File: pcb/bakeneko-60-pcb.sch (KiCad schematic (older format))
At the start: 17 parts, among them J1 JST SH 4-pin, SW1 Reset, U1 USBLC6-2SC6, U2 ATmega32U4-AU, Y1 16MHz

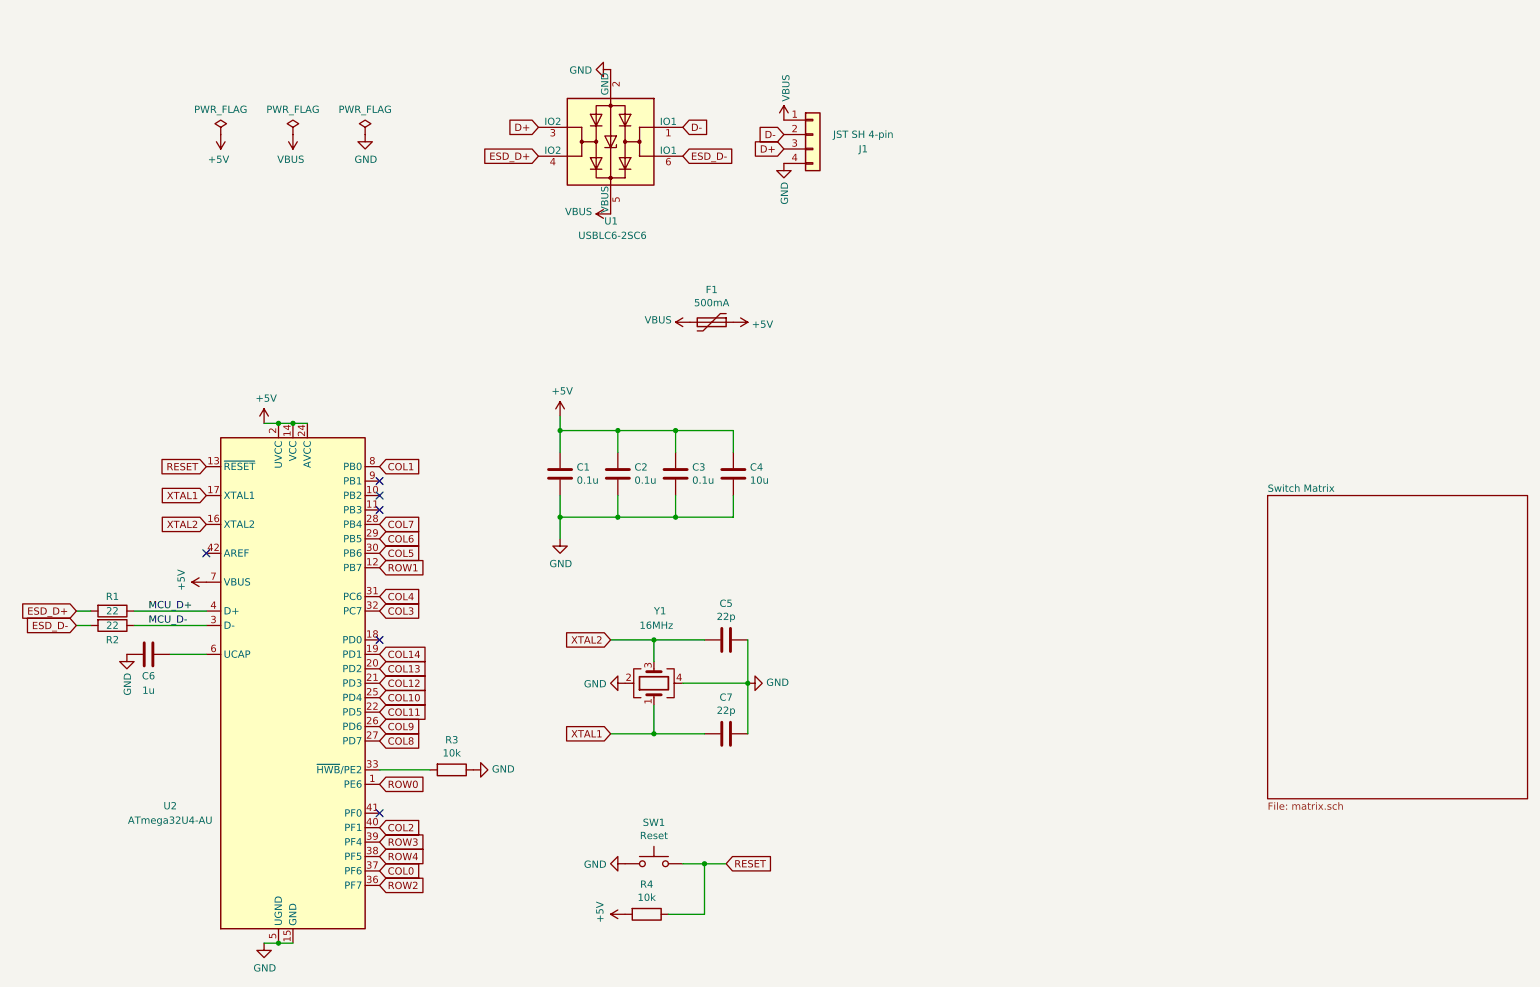
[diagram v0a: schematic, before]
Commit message: Update PCB
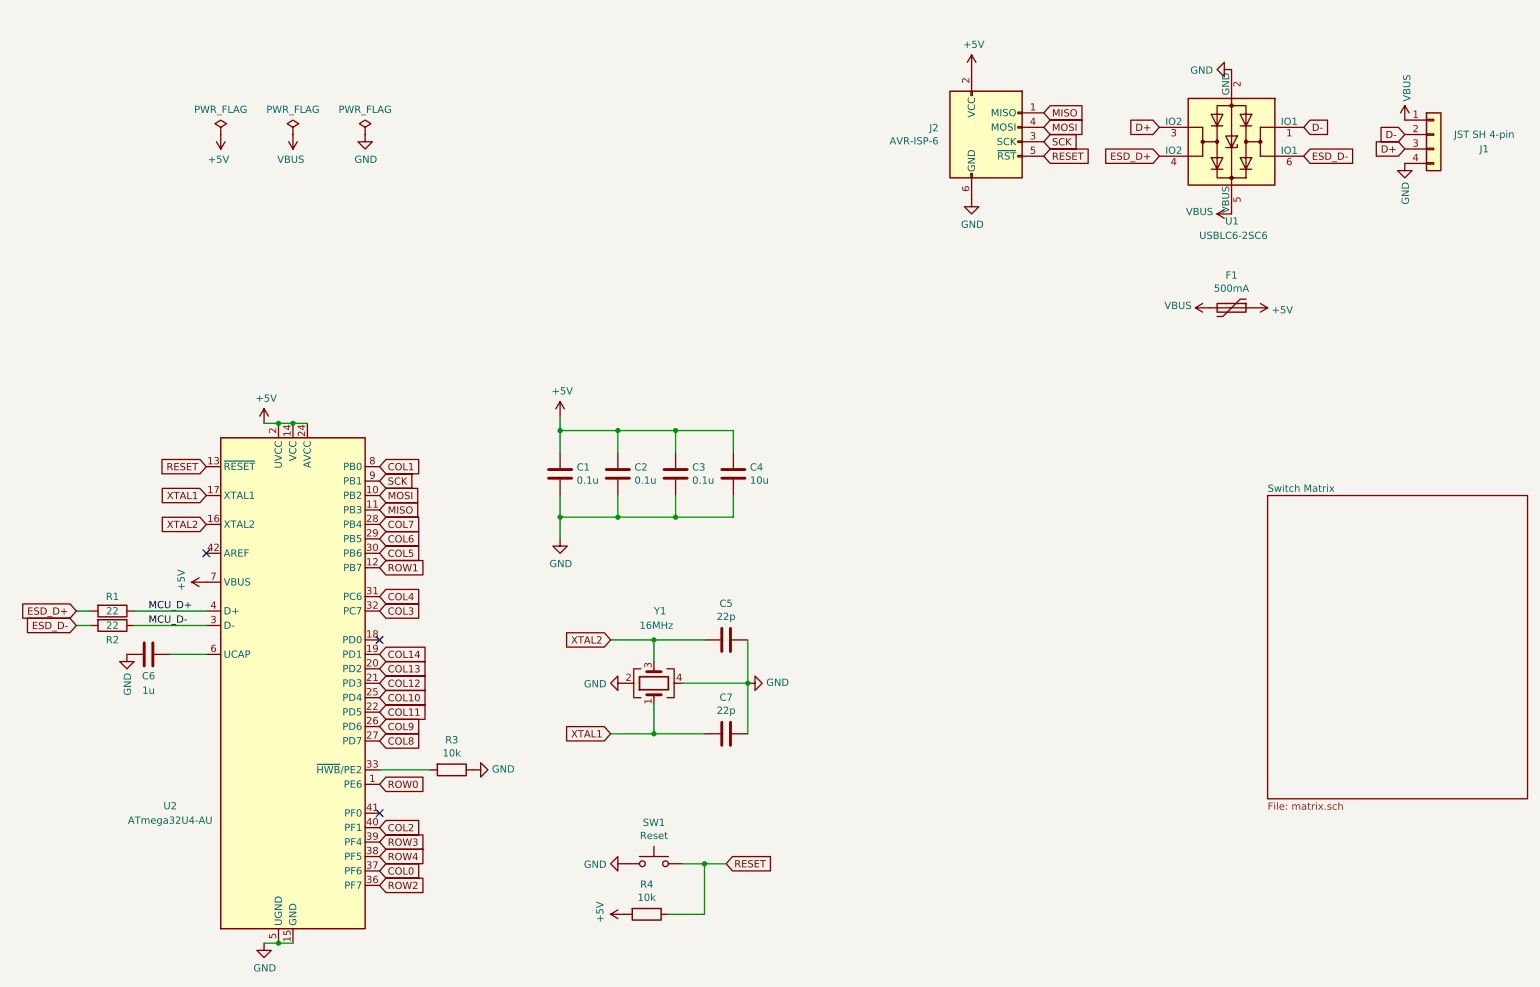
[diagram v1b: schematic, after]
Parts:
- added J2: AVR-ISP-6, random-keyboard-parts:Reset_Pretty, symbol Connector:AVR-ISP-6
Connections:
- net +5V: now also J2.2 (VCC)
- net GND: now also J2.6 (GND)
- net RESET: now also J2.5 (~RST)
- net MOSI: now reaches U2.10 (PB2)
- net MOSI: now also J2.4 (MOSI)
- net MISO: now reaches U2.11 (PB3)
- net MISO: now also J2.1 (MISO)
- net SCK: now reaches U2.9 (PB1)
- net SCK: now also J2.3 (SCK)
- no-connect marks 6 -> 3
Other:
- moved on the sheet: F1, J1, U1
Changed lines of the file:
@@
 encoding utf-8
 Sheet 1 2
-Title "Bakeneko 60"
+Title "Bakeneko 65"
 Date "2020-08-01"
-Rev "3.0"
+Rev "1"
 Comp ""
 Comment1 ""
@@
 L Device:Polyfuse F1
 U 1 1 5F2505EB
-P 5250 2900
-F 0 "F1" V 5025 2900 50  0000 C CNN
-F 1 "500mA" V 5116 2900 50  0000 C CNN
-F 2 "Fuse:Fuse_1206_3216Metric" H 5300 2700 50  0001 L CNN
-F 3 "~" H 5250 2900 50  0001 C CNN
-F 4 "C70076" H 5250 2900 50  0001 C CNN "LCSC Part #"
-	1    5250 2900
+P 8850 2800
+F 0 "F1" V 8625 2800 50  0000 C CNN
+F 1 "500mA" V 8716 2800 50  0000 C CNN
+F 2 "Fuse:Fuse_1206_3216Metric" H 8900 2600 50  0001 L CNN
+F 3 "~" H 8850 2800 50  0001 C CNN
+F 4 "C70076" H 8850 2800 50  0001 C CNN "LCSC Part #"
+	1    8850 2800
 	0    1    1    0
 $EndComp
@@
 L Connector_Generic:Conn_01x04 J1
 U 1 1 5F252816
-P 5950 1600
-F 0 "J1" H 6300 1500 50  0000 C CNN
-F 1 "JST SH 4-pin" H 6300 1600 50  0000 C CNN
-F 2 "Connector_JST:JST_SH_SM04B-SRSS-TB_1x04-1MP_P1.00mm_Horizontal" H 5950 1600 50  0001 C CNN
-F 3 "~" H 5950 1600 50  0001 C CNN
-F 4 "C160404" H 5950 1600 50  0001 C CNN "LCSC Part #"
-	1    5950 1600
+P 10250 1600
+F 0 "J1" H 10600 1500 50  0000 C CNN
+F 1 "JST SH 4-pin" H 10600 1600 50  0000 C CNN
+F 2 "Connector_JST:JST_SH_SM04B-SRSS-TB_1x04-1MP_P1.00mm_Horizontal" H 10250 1600 50  0001 C CNN
+F 3 "~" H 10250 1600 50  0001 C CNN
+F 4 "C160404" H 10250 1600 50  0001 C CNN "LCSC Part #"
+	1    10250 1600
 	1    0    0    -1
 $EndComp
@@
 L power:GND #PWR02
 U 1 1 5F256D2D
-P 4550 1150
-F 0 "#PWR02" H 4550 900 50  0001 C CNN
-F 1 "GND" V 4555 1022 50  0000 R CNN
-F 2 "" H 4550 1150 50  0001 C CNN
-F 3 "" H 4550 1150 50  0001 C CNN
-	1    4550 1150
+P 8850 1150
+F 0 "#PWR02" H 8850 900 50  0001 C CNN
+F 1 "GND" V 8855 1022 50  0000 R CNN
+F 2 "" H 8850 1150 50  0001 C CNN
+F 3 "" H 8850 1150 50  0001 C CNN
+	1    8850 1150
 	0    1    1    0
 $EndComp
@@
 	0    1    1    0
 $EndComp
-Text GLabel 5750 1600 0    50   Input ~ 0
+Text GLabel 10050 1600 0    50   Input ~ 0
 D-
-Text GLabel 5750 1700 0    50   Input ~ 0
+Text GLabel 10050 1700 0    50   Input ~ 0
 D+
 $Comp
@@
 L power:VBUS #PWR03
 U 1 1 5F275D18
-P 5750 1500
-F 0 "#PWR03" H 5750 1350 50  0001 C CNN
-F 1 "VBUS" V 5765 1628 50  0000 L CNN
-F 2 "" H 5750 1500 50  0001 C CNN
-F 3 "" H 5750 1500 50  0001 C CNN
-	1    5750 1500
+P 10050 1500
+F 0 "#PWR03" H 10050 1350 50  0001 C CNN
+F 1 "VBUS" V 10065 1628 50  0000 L CNN
+F 2 "" H 10050 1500 50  0001 C CNN
+F 3 "" H 10050 1500 50  0001 C CNN
+	1    10050 1500
 	1    0    0    -1
 $EndComp
@@
 L power:VBUS #PWR09
 U 1 1 5F276E32
-P 4550 2150
-F 0 "#PWR09" H 4550 2000 50  0001 C CNN
-F 1 "VBUS" V 4565 2278 50  0000 L CNN
-F 2 "" H 4550 2150 50  0001 C CNN
-F 3 "" H 4550 2150 50  0001 C CNN
-	1    4550 2150
+P 8850 2150
+F 0 "#PWR09" H 8850 2000 50  0001 C CNN
+F 1 "VBUS" V 8865 2278 50  0000 L CNN
+F 2 "" H 8850 2150 50  0001 C CNN
+F 3 "" H 8850 2150 50  0001 C CNN
+	1    8850 2150
 	0    -1   -1   0
 $EndComp
@@
 L power:VBUS #PWR010
 U 1 1 5F277A1C
-P 5100 2900
-F 0 "#PWR010" H 5100 2750 50  0001 C CNN
-F 1 "VBUS" V 5115 3027 50  0000 L CNN
-F 2 "" H 5100 2900 50  0001 C CNN
-F 3 "" H 5100 2900 50  0001 C CNN
-	1    5100 2900
+P 8700 2800
+F 0 "#PWR010" H 8700 2650 50  0001 C CNN
+F 1 "VBUS" V 8715 2927 50  0000 L CNN
+F 2 "" H 8700 2800 50  0001 C CNN
+F 3 "" H 8700 2800 50  0001 C CNN
+	1    8700 2800
 	0    -1   -1   0
 $EndComp
-Text GLabel 4050 1550 0    50   Input ~ 0
+Text GLabel 8350 1550 0    50   Input ~ 0
 D+
-Text GLabel 5050 1550 2    50   Input ~ 0
+Text GLabel 9350 1550 2    50   Input ~ 0
 D-
 $Comp
@@
 Wire Wire Line
 	5050 5400 5500 5400
+$Comp
+L Connector:AVR-ISP-6 J2
+U 1 1 5F4C9CCE
+P 7150 1650
+F 0 "J2" H 6821 1746 50  0000 R CNN
+F 1 "AVR-ISP-6" H 6821 1655 50  0000 R CNN
+F 2 "random-keyboard-parts:Reset_Pretty" V 6900 1700 50  0001 C CNN
+F 3 " ~" H 5875 1100 50  0001 C CNN
+	1    7150 1650
+	1    0    0    -1
+$EndComp
+$Comp
+L power:GND #PWR08
+U 1 1 5F4D2BF6
+P 7050 2050
+F 0 "#PWR08" H 7050 1800 50  0001 C CNN
+F 1 "GND" H 7055 1877 50  0000 C CNN
+F 2 "" H 7050 2050 50  0001 C CNN
+F 3 "" H 7050 2050 50  0001 C CNN
+	1    7050 2050
+	1    0    0    -1
+$EndComp
+Text GLabel 7550 1450 2    50   Input ~ 0
+MISO
+Text GLabel 7550 1550 2    50   Input ~ 0
+MOSI
+Text GLabel 7550 1650 2    50   Input ~ 0
+SCK
+Text GLabel 7550 1750 2    50   Input ~ 0
+RESET
+Text GLabel 2950 4200 2    50   Input ~ 0
+MISO
+Text GLabel 2950 4000 2    50   Input ~ 0
+SCK
+Text GLabel 2950 4100 2    50   Input ~ 0
+MOSI
 Text GLabel 2950 5200 2    50   Input ~ 0
 COL14
@@
 L Power_Protection:USBLC6-2SC6 U1
 U 1 1 5F25444E
-P 4550 1650
-F 0 "U1" H 4500 2200 50  0000 L CNN
-F 1 "USBLC6-2SC6" H 4300 2300 50  0000 L CNN
-F 2 "Package_TO_SOT_SMD:SOT-23-6" H 4550 1150 50  0001 C CNN
-F 3 "https://www.st.com/resource/en/datasheet/usblc6-2.pdf" H 4750 2000 50  0001 C CNN
-F 4 "C7519" H 4550 1650 50  0001 C CNN "LCSC Part #"
-	1    4550 1650
+P 8850 1650
+F 0 "U1" H 8800 2200 50  0000 L CNN
+F 1 "USBLC6-2SC6" H 8600 2300 50  0000 L CNN
+F 2 "Package_TO_SOT_SMD:SOT-23-6" H 8850 1150 50  0001 C CNN
+F 3 "https://www.st.com/resource/en/datasheet/usblc6-2.pdf" H 9050 2000 50  0001 C CNN
+F 4 "C7519" H 8850 1650 50  0001 C CNN "LCSC Part #"
+	1    8850 1650
 	-1   0    0    1
 $EndComp
@@
 L power:GND #PWR07
 U 1 1 5F253A4B
-P 5750 1800
-F 0 "#PWR07" H 5750 1550 50  0001 C CNN
-F 1 "GND" V 5755 1672 50  0000 R CNN
-F 2 "" H 5750 1800 50  0001 C CNN
-F 3 "" H 5750 1800 50  0001 C CNN
-	1    5750 1800
+P 10050 1800
+F 0 "#PWR07" H 10050 1550 50  0001 C CNN
+F 1 "GND" V 10055 1672 50  0000 R CNN
+F 2 "" H 10050 1800 50  0001 C CNN
+F 3 "" H 10050 1800 50  0001 C CNN
+	1    10050 1800
 	1    0    0    -1
 $EndComp
@@
 Wire Wire Line
 	850  4900 950  4900
-Text GLabel 5050 1750 2    50   Input ~ 0
+Text GLabel 9350 1750 2    50   Input ~ 0
 ESD_D-
-Text GLabel 4050 1750 0    50   Input ~ 0
+Text GLabel 8350 1750 0    50   Input ~ 0
 ESD_D+
 $Comp
@@
 L power:+5V #PWR011
 U 1 1 5F3C7287
-P 5400 2900
-F 0 "#PWR011" H 5400 2750 50  0001 C CNN
-F 1 "+5V" V 5415 3028 50  0000 L CNN
-F 2 "" H 5400 2900 50  0001 C CNN
-F 3 "" H 5400 2900 50  0001 C CNN
-	1    5400 2900
-	0    1    1    0
+P 9000 2800
+F 0 "#PWR011" H 9000 2650 50  0001 C CNN
+F 1 "+5V" V 9015 2928 50  0000 L CNN
+F 2 "" H 9000 2800 50  0001 C CNN
+F 3 "" H 9000 2800 50  0001 C CNN
+	1    9000 2800
+	0    1    1    0
+$EndComp
+$Comp
+L power:+5V #PWR01
+U 1 1 5F3D1A13
+P 7050 1150
+F 0 "#PWR01" H 7050 1000 50  0001 C CNN
+F 1 "+5V" H 7065 1323 50  0000 C CNN
+F 2 "" H 7050 1150 50  0001 C CNN
+F 3 "" H 7050 1150 50  0001 C CNN
+	1    7050 1150
+	1    0    0    -1
 $EndComp
 $Comp
@@
 ROW3
 NoConn ~ 2950 5100
-NoConn ~ 2950 4200
-NoConn ~ 2950 4100
-NoConn ~ 2950 4000
 $EndSCHEMATC
